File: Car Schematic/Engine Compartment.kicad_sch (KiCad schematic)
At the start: 8 parts

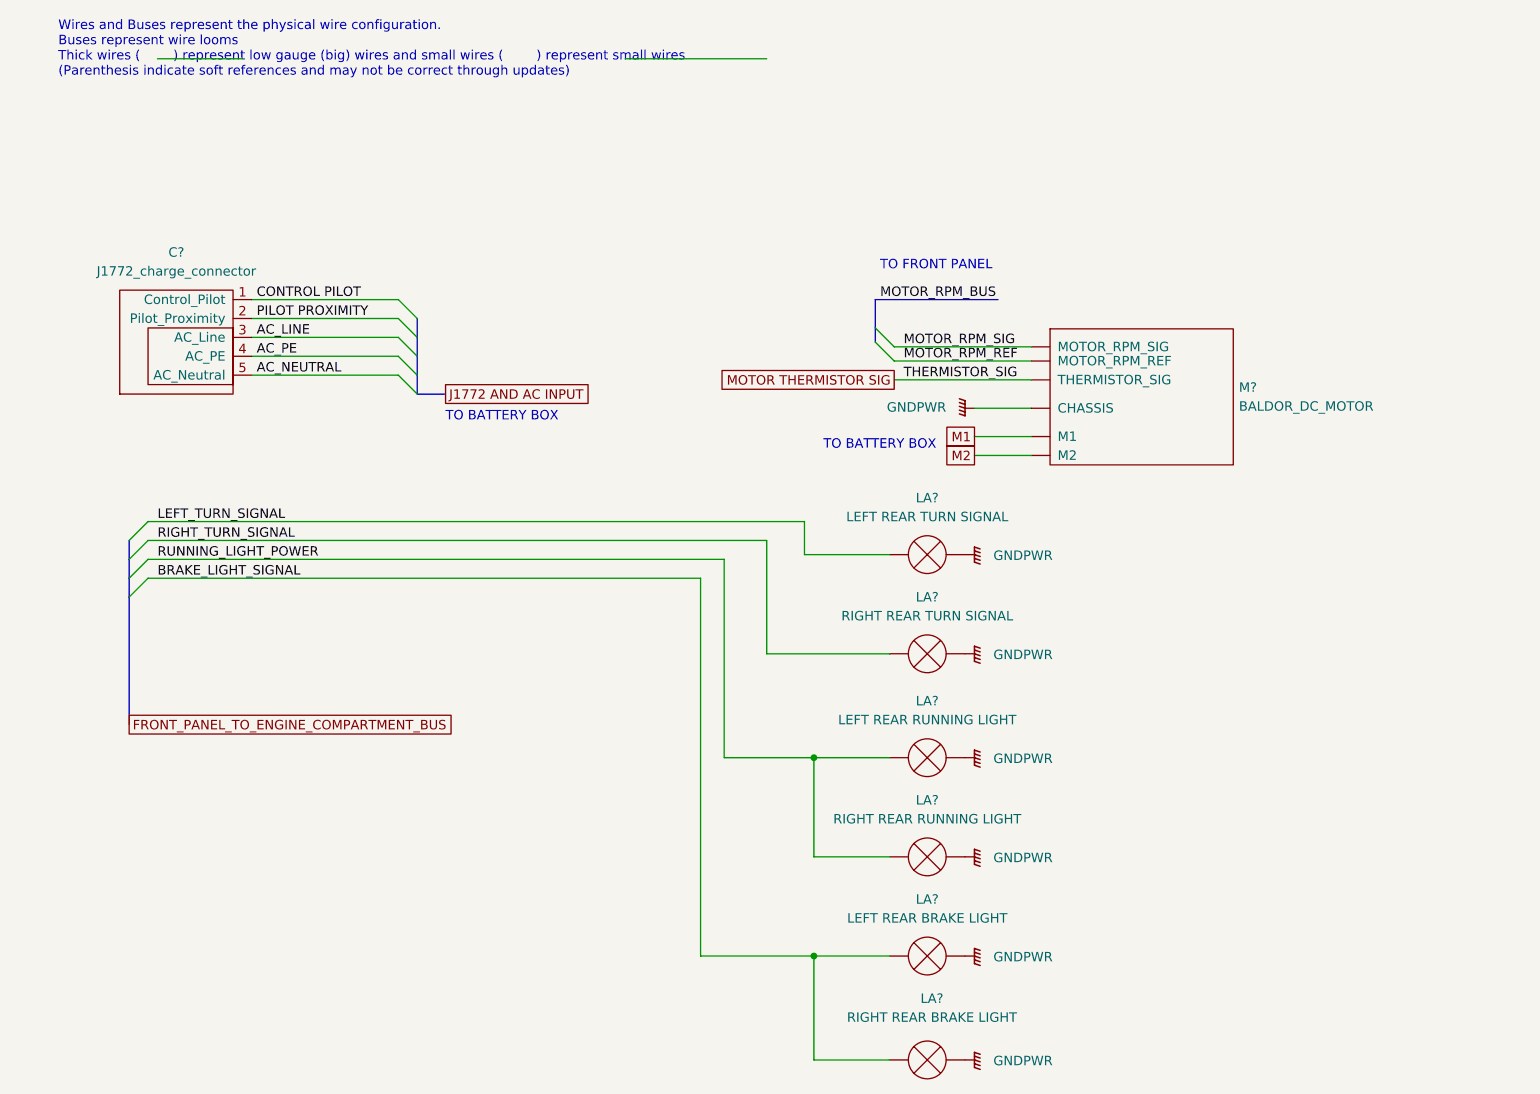
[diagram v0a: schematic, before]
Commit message: updating more things!
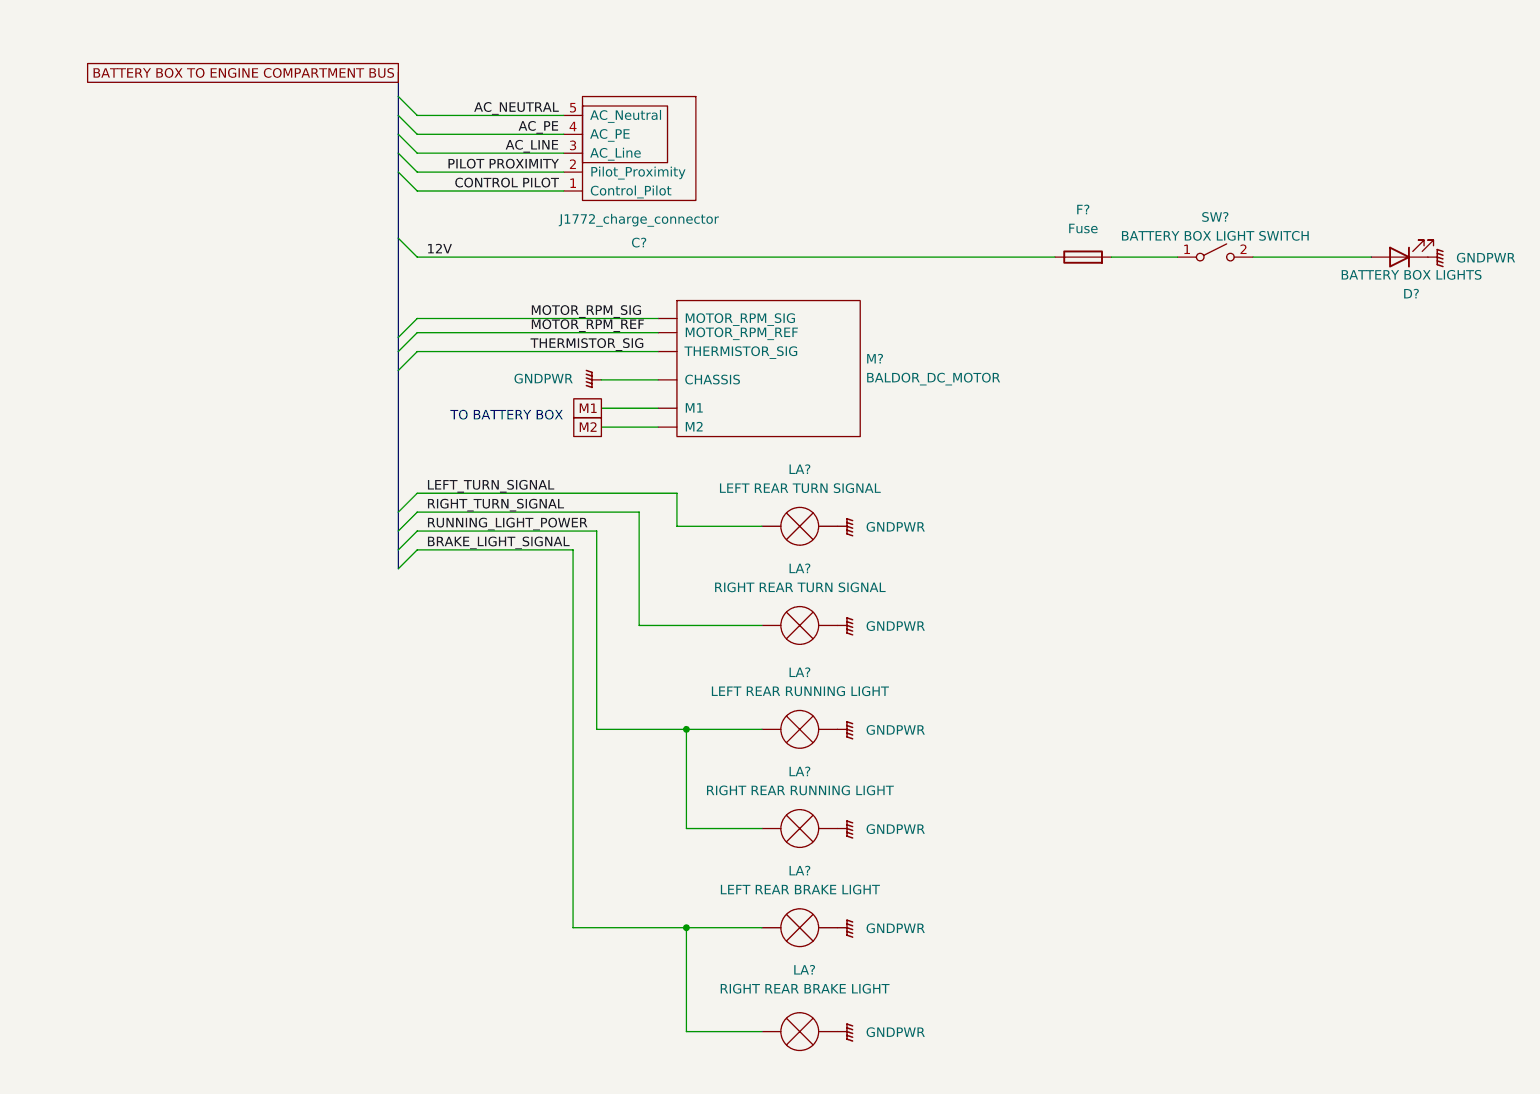
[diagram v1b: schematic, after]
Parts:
- added D?: BATTERY BOX LIGHTS, symbol Device:LED
- added F?: Fuse, symbol Device:Fuse
- added SW?: BATTERY BOX LIGHT SWITCH, symbol Switch:SW_SPST
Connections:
- net GNDPWR: now also D?.1 (K)
- net MOTOR THERMISTOR SIG renamed THERMISTOR_SIG
- new net: F?.2, SW?.1 (A)
- new net: D?.2 (A), SW?.2 (B)
- new net 12V: F?.1
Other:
- note removed: "TO FRONT PANEL"
- note removed: "Wires and Buses represent the physical wire configuration. Buses represent wire looms Thick wires ( ) represent low gauge (big) wires and small wires ( ) represent small wires (Parenthesis indicate soft references and may not be correct through updates)"
- moved on the sheet: C?, LA?, M?
